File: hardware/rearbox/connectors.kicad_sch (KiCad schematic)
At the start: 2 parts, among them J3 Conn_02x28_Top_Bottom, J4 Auxiliary

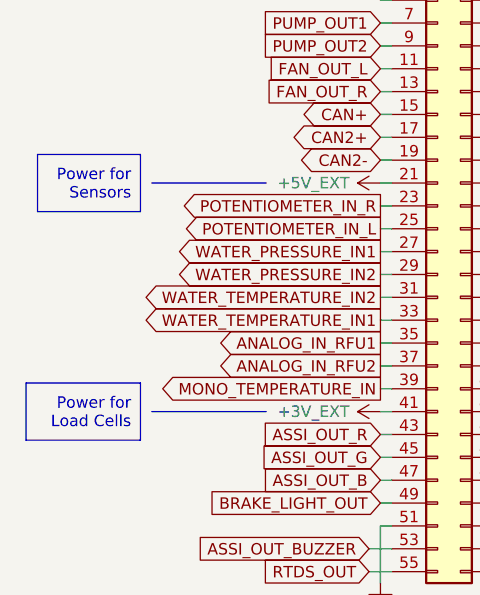
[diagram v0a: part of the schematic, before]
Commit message: Changed power section
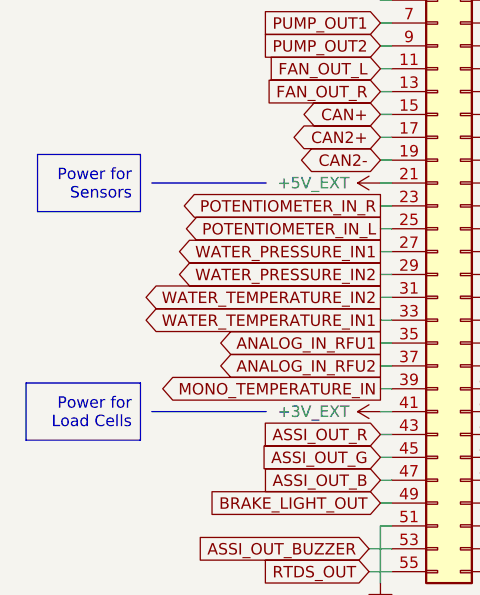
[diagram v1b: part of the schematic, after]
